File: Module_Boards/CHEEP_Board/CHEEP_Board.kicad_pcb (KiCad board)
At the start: 6 copper layers, 17.5 x 26.4 mm, 53 parts, among them U2 HEEPocrates, U3 SIT1532AC-J5-DCC-32.768D, U4 W25Q128JWYIQ

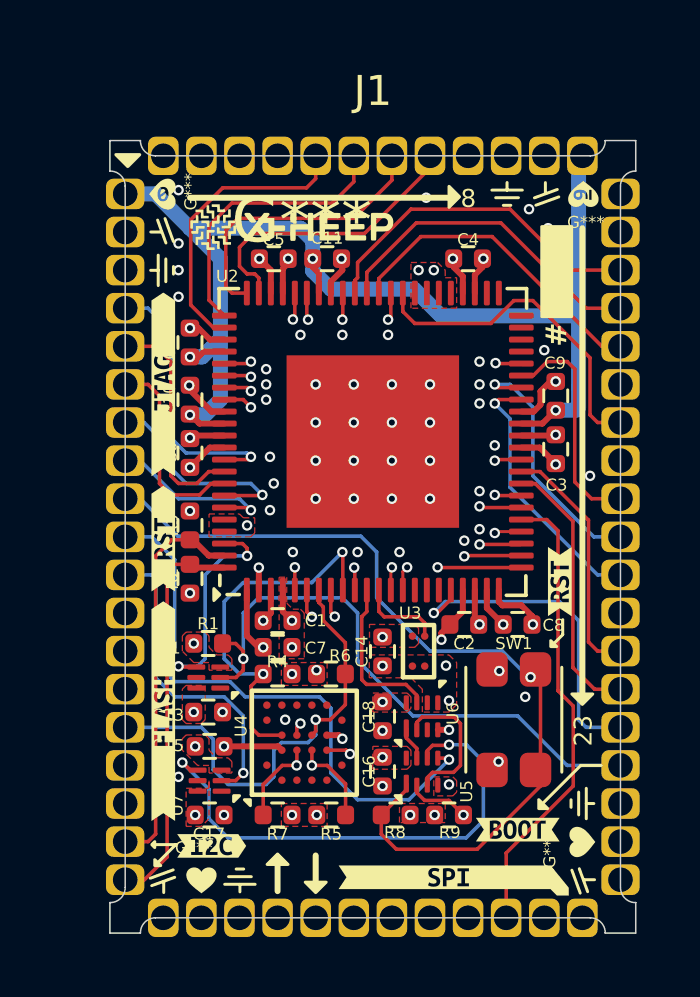
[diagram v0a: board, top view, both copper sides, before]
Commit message: Big push. Fixed the issues that were pending. See github
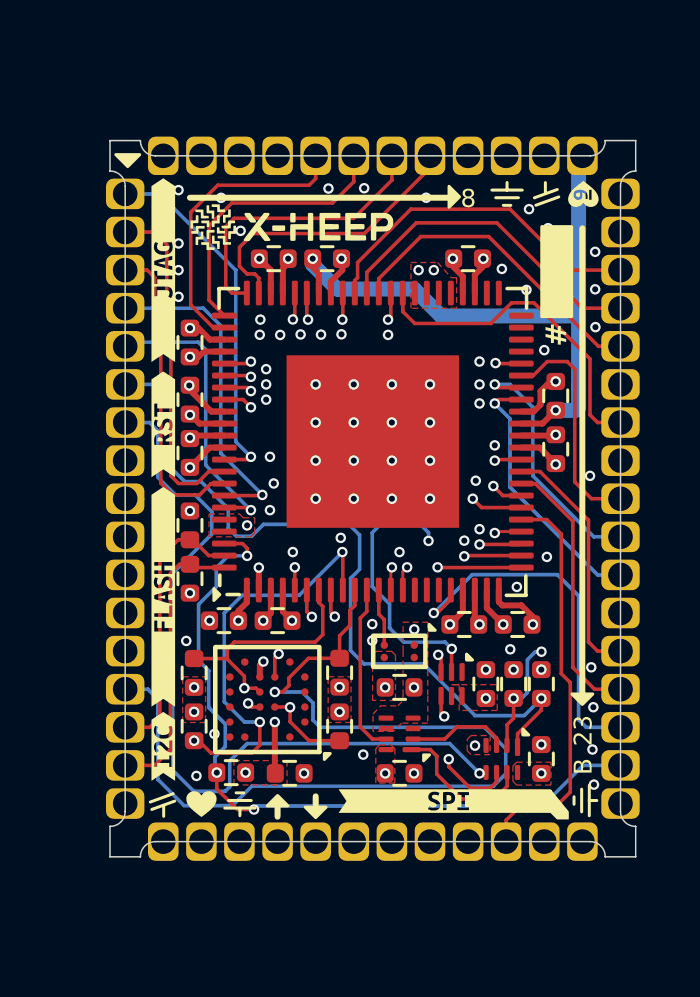
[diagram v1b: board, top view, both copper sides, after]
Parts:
- removed C13: 100n 10V, X-MODs_PcbLib:C0402
- removed the G*** at (113.5, 114.6)
- removed the G*** at (101.5, 92.6)
- removed SW1: ~, X-MODs_PcbLib:TL1030AF160AQJ
- removed U1: ~, X-MODs_PcbLib:X2SON-6
- removed kibuzzard-67265B69: G***, kibuzzard-67265B69
- removed kibuzzard-67265C69: G***, kibuzzard-67265C69
- R1: value 100K -> 10K0
- moved C17 10.2 mm to (111.3, 109.0), turned to -90 degrees
- moved U7 8.68 mm to (110.2, 109.0), turned to -90 degrees
- moved R8 6.53 mm to (113.2, 109.0), turned to -90 degrees
- moved C16 5.31 mm to (113.2, 111.5), turned to -90 degrees
- moved R9 4.87 mm to (112.3, 109.0), turned to -90 degrees
- moved R5 4.75 mm to (106.5, 108.7), turned to 90 degrees
- moved R6 4.56 mm to (101.6, 108.7), turned to 90 degrees
- moved R1 4.37 mm to (102.8, 112.0)
- moved kibuzzard-67265A85 3.81 mm to (100.6, 95.2)
- moved kibuzzard-67265AAD 3.81 mm to (100.6, 100.4)
- moved kibuzzard-67265ADF 3.81 mm to (100.6, 106.1)
- moved kibuzzard-67265AFB 3.69 mm to (100.6, 111.1), turned to 90 degrees
- moved R7 3.61 mm to (106.5, 110.5), turned to -90 degrees
- moved R4 3.28 mm to (101.6, 110.5), turned to -90 degrees
- moved C15 2.82 mm to (104.8, 112.0), turned to 180 degrees
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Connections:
- J1 pad 1: VCORE -> JTAG_TDO
- J1 pad 10: PMIC_nRST -> FLASH_MISO
- J1 pad 11: SOC_RST_OUT -> FLASH_CS
- J1 pad 12: FLASH_MOSI -> FLASH_nWP
- J1 pad 13: FLASH_MISO -> FLASH_nHLD_nRST
- J1 pad 14: FLASH_CS -> FLASH_SCK
- J1 pad 15: FLASH_nWP -> I2C_SDA_HEEP
- J1 pad 16: FLASH_nHLD_nRST -> I2C_SCL_HEEP
- J1 pad 17: FLASH_SCK -> GND
- J1 pad 18: I2C_SDA_HEEP -> +1V8
- J1 pad 19: I2C_SCL_HEEP -> VCORE
- J1 pad 2: +1V8 -> JTAG_TDI
- J1 pad 20: +1V8 -> GND
- J1 pad 21: VCORE -> UART_RX_HEEP
- J1 pad 22: GND -> UART_TX_HEEP
- J1 pad 23: UART_RX_HEEP -> SPI_MOSI_HEEP
- J1 pad 24: UART_TX_HEEP -> SPI_MISO_HEEP
- J1 pad 25: SPI_MOSI_HEEP -> SPI_SD2_HEEP
- J1 pad 26: SPI_MISO_HEEP -> SPI_SD3_HEEP
- J1 pad 27: SPI_SD2_HEEP -> SPI_CS1_HEEP
- J1 pad 28: SPI_SD3_HEEP -> SPI_CS0_HEEP
- J1 pad 29: SPI_CS1_HEEP -> SPI_SCK_HEEP
- J1 pad 3: GND -> JTAG_TRST
- J1 pad 30: SPI_CS0_HEEP -> GND
- J1 pad 31: SPI_SCK_HEEP -> BOOT_SEL_EXT
- J1 pad 32: +1V8 -> GPIO_23
- J1 pad 33: VCORE -> GPIO_22
- J1 pad 34: GND -> GPIO_21
- J1 pad 35: BOOT_SEL_EXT -> GPIO_20
- J1 pad 36: GPIO_23 -> GPIO_19
- J1 pad 37: GPIO_22 -> GPIO_18
- J1 pad 38: GPIO_21 -> GPIO_17
- J1 pad 39: GPIO_20 -> GPIO_16
- J1 pad 4: JTAG_TDO -> JTAG_TMS
- J1 pad 40: GPIO_19 -> GPIO_15
- J1 pad 41: GPIO_18 -> GPIO_14
- J1 pad 42: GPIO_17 -> GPIO_13
- J1 pad 43: GPIO_16 -> GPIO_12
- J1 pad 44: GPIO_15 -> GPIO_11
- J1 pad 45: GPIO_14 -> GPIO_10
- J1 pad 46: GPIO_13 -> GPIO_9
- J1 pad 47: GPIO_12 -> VCORE
- J1 pad 48: GPIO_11 -> +1V8
- J1 pad 49: GPIO_10 -> GND
- J1 pad 5: JTAG_TDI -> JTAG_TCK
- J1 pad 50: GPIO_9 -> GPIO_8
- J1 pad 51: VCORE -> GPIO_7
- J1 pad 52: +1V8 -> GPIO_6
- J1 pad 53: GND -> GPIO_5
- J1 pad 54: GPIO_8 -> GPIO_4
- J1 pad 55: GPIO_7 -> GPIO_3
- J1 pad 56: GPIO_6 -> GPIO_2
- J1 pad 57: GPIO_5 -> GPIO_1
- J1 pad 58: GPIO_4 -> GPIO_0
- J1 pad 6: JTAG_TRST -> Manual_RST
- J1 pad 7: JTAG_TMS -> PMIC_nRST
- J1 pad 8: JTAG_TCK -> SOC_RST_OUT
- J1 pad 9: Manual_RST -> FLASH_MOSI
- R1 pad 1: BOOT_SEL_EXT -> +1V8
- R1 pad 2: GND -> BOOT_SEL_EXT
- U2 pad 86: /[1] HEEPocrates/BOOT_SELECT -> BOOT_SEL_EXT
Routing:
- net VCORE: track 83.4 -> 63.2 mm
- net /[2] Connectors & Flash/nSOC_RST: track 16.9 -> 4.75 mm
- net FLASH_SCK: track 20.0 -> 31.2 mm, vias 2 -> 1
- net SOC_RST_OUT: track 10.6 -> 20.4 mm, vias 1 -> 2
- net JTAG_TRST: track 33.0 -> 40.3 mm, vias 1 -> 2
- net /[1] HEEPocrates/BOOT_SELECT: track 7.13 -> 0.00 mm, vias 2 -> 0
- net PMIC_nRST: track 19.2 -> 26.3 mm
- net BOOT_SEL_EXT: track 19.8 -> 24.8 mm, vias 1 -> 3
- net I2C_SDA_HEEP: track 13.1 -> 8.96 mm
- net FLASH_CS: track 17.2 -> 21.2 mm, vias 2 -> 3
- net JTAG_TCK: track 5.80 -> 9.75 mm
- net Manual_RST: track 29.2 -> 25.3 mm
- net JTAG_TDI: track 7.60 -> 11.4 mm
- net I2C_SCL_HEEP: track 13.3 -> 9.57 mm
- net /[2] Connectors & Flash/RST_A: track 1.14 -> 4.85 mm
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- added copper zone on In3.Cu, net GND
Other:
- board size 17.5 x 26.4 mm -> 17.5 x 23.9 mm
- board text added: "B"
